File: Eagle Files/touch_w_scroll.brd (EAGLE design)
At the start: 160 x 100 mm, 8 parts

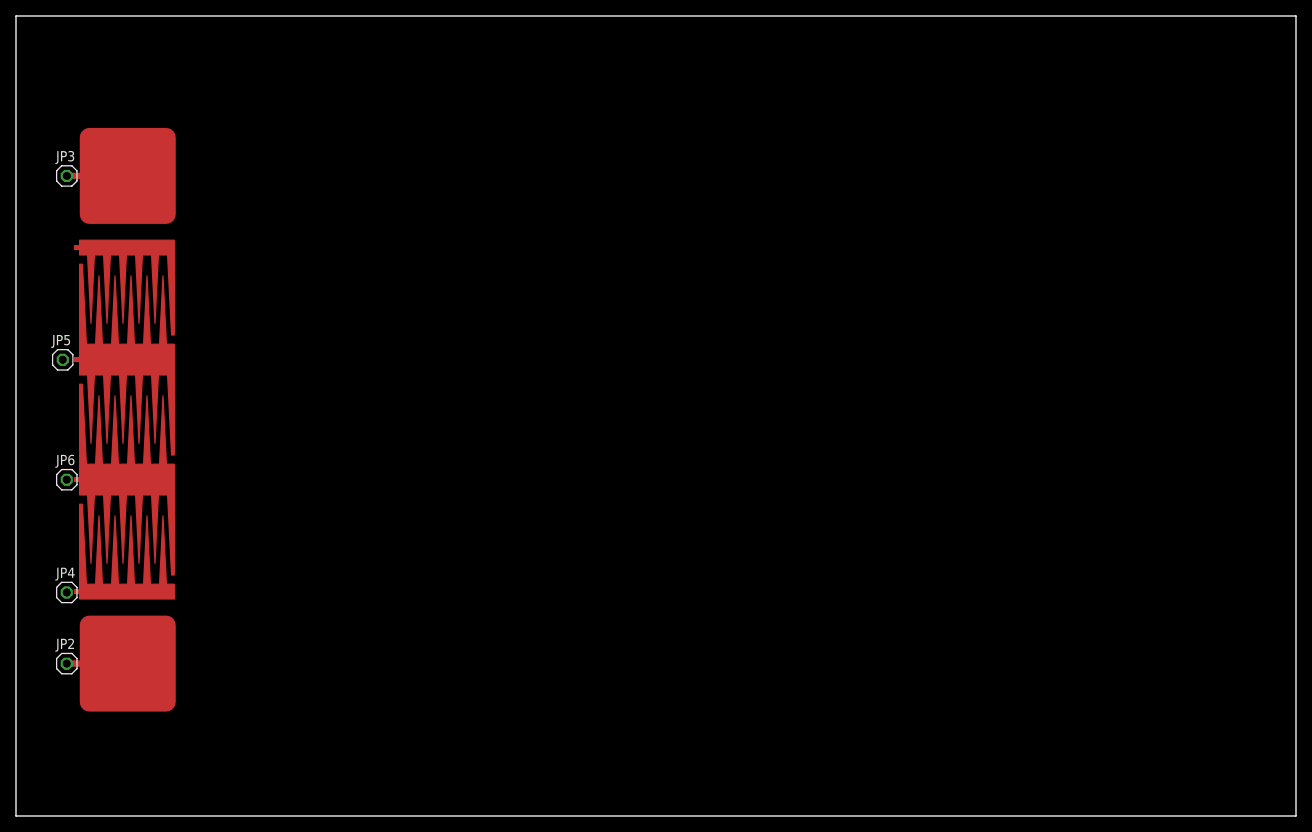
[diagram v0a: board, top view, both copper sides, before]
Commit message: updates
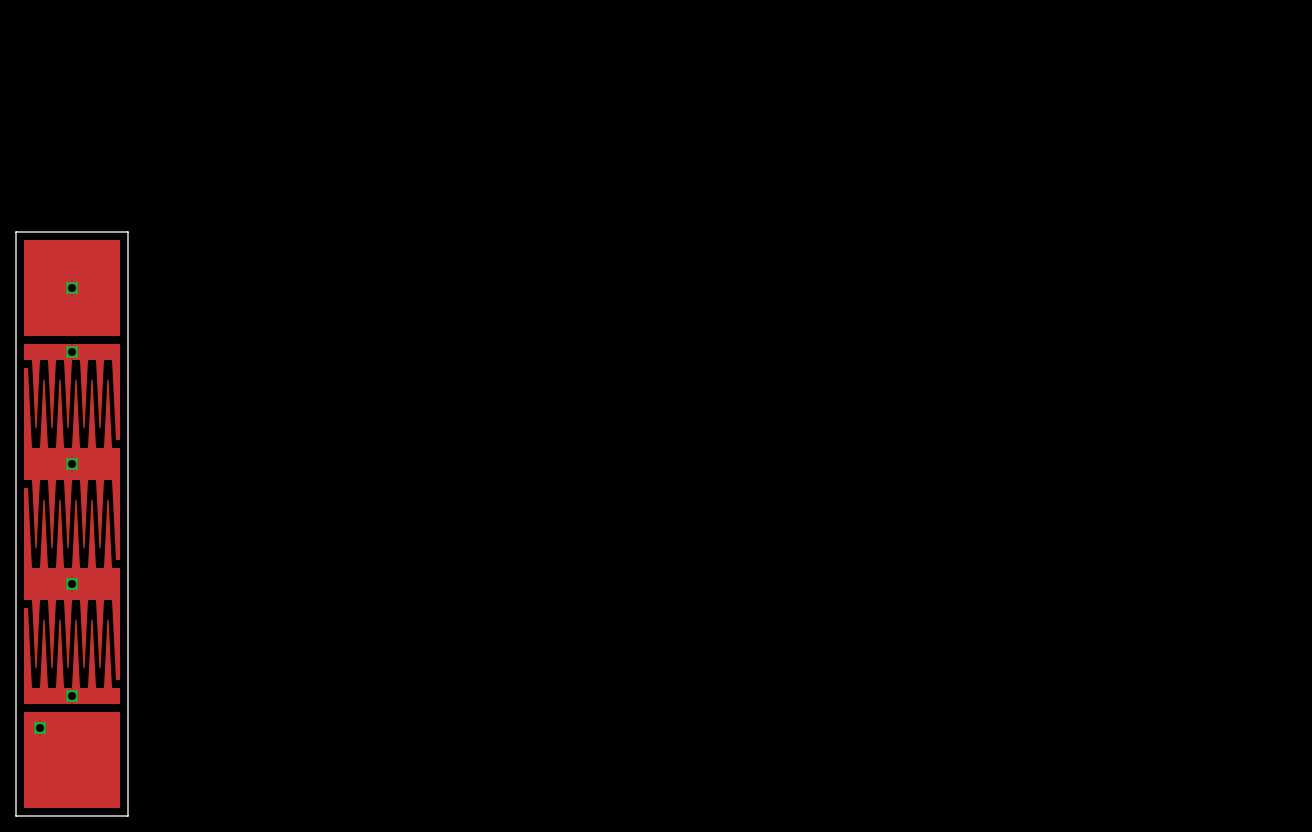
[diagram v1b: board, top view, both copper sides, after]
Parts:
- removed JP2, JP3, JP4, JP5, JP6: PINHD-1X1, Connector:1X01
- removed U$3: 12X12_PAD, Cap Touch Pads:12X12_PAD
- added U$4: 12X12_PADLED, Cap Touch Pads:12X12_PAD_LED
- moved U$2 54.5 mm to (1.00, 72.0)
- moved U$1 32.4 mm to (13.0, 59.0), turned to 270 degrees
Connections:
- removed net N$1: JP3.1, U$3.1
- removed net N$2: JP4.1, U$1.1, U$1.4
- removed net N$3: JP5.1, U$1.3
- removed net N$4: JP6.1, U$1.2
- removed net N$5: JP2.1, U$2.1
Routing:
- net N$5: track 7.62 -> 0.00 mm
- net N$1: track 7.62 -> 0.00 mm
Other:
- board size 160 x 100 mm -> 14 x 73 mm
